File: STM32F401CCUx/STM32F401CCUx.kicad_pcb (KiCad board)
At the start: 2 copper layers, 46 x 64.5 mm, 60 parts, among them J1 Conn_01x04, J2 Power_Conn, J3 SWD, J4 USB_C_Receptacle_USB2.0, Q1 AO3401A, SW1 SW_SPDT, U1 MSM38A2718Z9BM3, U2 EUP3458, U3 LM321, U4 STM32F401CCUx, U5 USBLC6-2SC6, Y1 25MHz

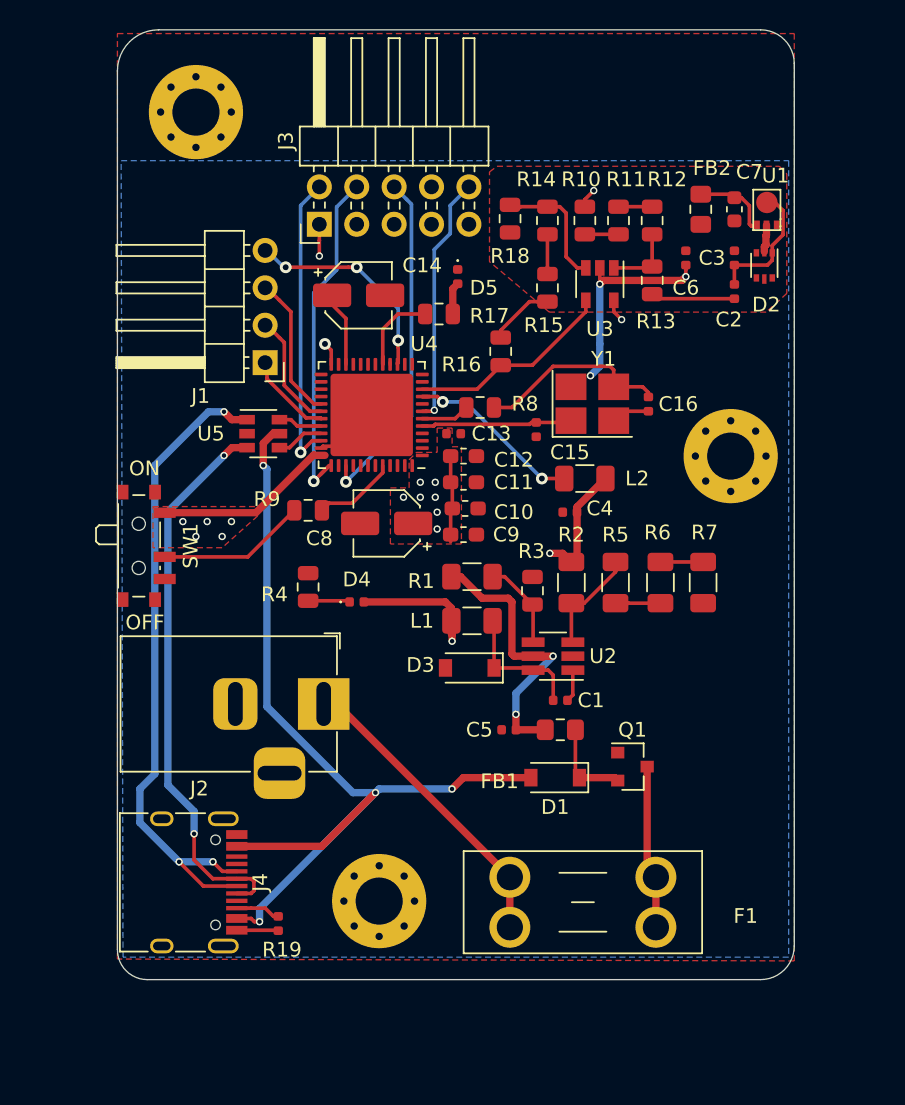
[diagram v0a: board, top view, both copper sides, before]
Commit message: Updated PCB
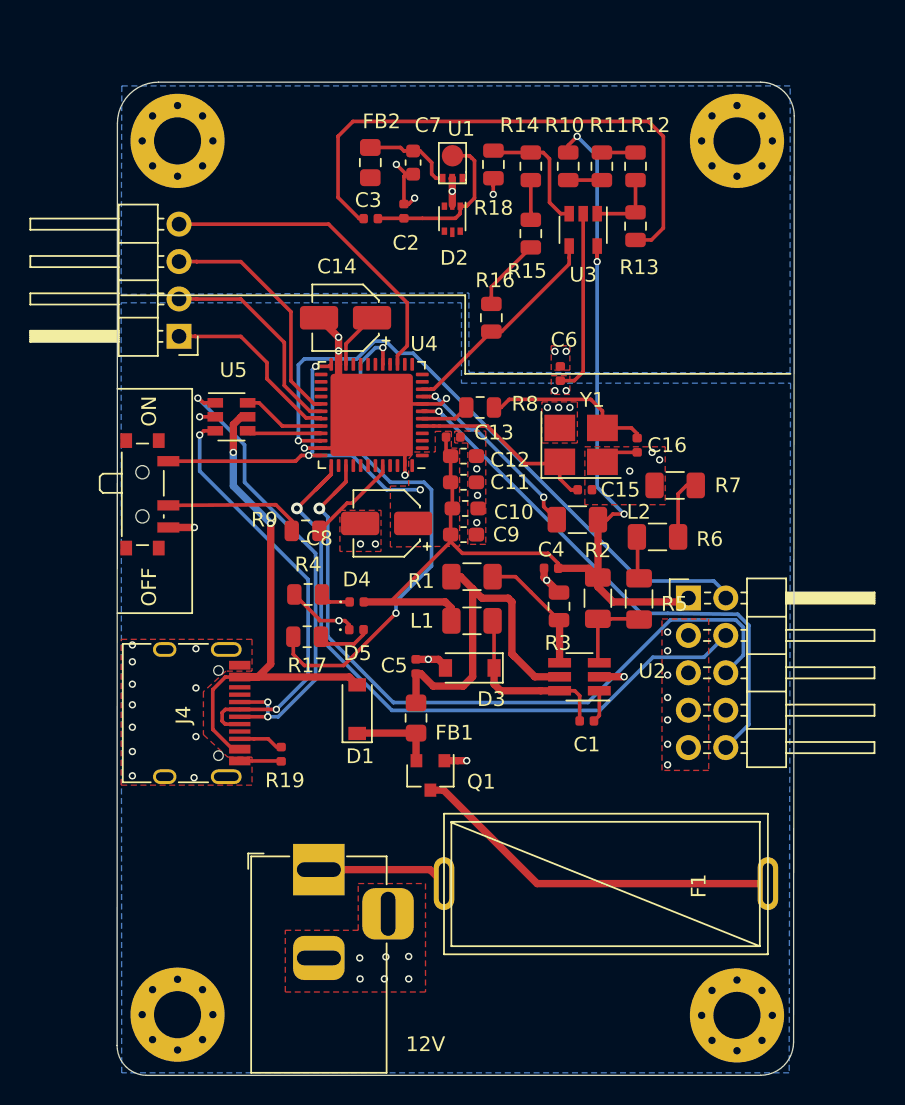
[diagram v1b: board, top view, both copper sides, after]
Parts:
- removed the REF** at (95.2, 82.0)
- removed the REF** at (131.6, 105.4)
- removed the REF** at (107.7, 135.6)
- added REF**: MountingHole_3.2mm_M3_Pad_Via, MountingHole:MountingHole_3.2mm_M3_Pad_Via, F.Cu at (94.0, 143.3)
- added REF**: MountingHole_3.2mm_M3_Pad_Via, MountingHole:MountingHole_3.2mm_M3_Pad_Via, F.Cu at (132.0, 143.4)
- added REF**: MountingHole_3.2mm_M3_Pad_Via, MountingHole:MountingHole_3.2mm_M3_Pad_Via, F.Cu at (132.0, 84.0)
- added REF**: MountingHole_3.2mm_M3_Pad_Via, MountingHole:MountingHole_3.2mm_M3_Pad_Via, F.Cu at (94.0, 84.0)
- F1: footprint Fuse:Fuseholder_Blade_Mini_Keystone_3568 -> Fuse_holder:FUSE-TH_L22.6-W9.0
- moved J3 35.7 mm to (128.7, 115.0), turned to 0 degrees
- moved C2 25.2 mm to (107.1, 89.3), turned to 0 degrees
- moved D5 24.9 mm to (106.2, 117.2), turned to 0 degrees
- moved R17 23.7 mm to (102.8, 117.7)
- moved FB2 22.7 mm to (107.1, 85.5)
- moved C3 22.7 mm to (109.4, 88.8)
- moved C7 22.1 mm to (110.0, 85.5)
- moved U1 21.6 mm to (113.6, 84.1)
- moved D2 21.4 mm to (112.7, 89.3)
- moved D1 14.2 mm to (106.2, 122.6), turned to 90 degrees
- moved Q1 13.7 mm to (111.2, 127.1), turned to 270 degrees
- moved C6 11.6 mm to (120.0, 99.8)
- moved J4 11.5 mm to (94.2, 122.9)
- moved R19 11.5 mm to (101.0, 125.7)
- moved J2 11.3 mm to (103.6, 133.5), turned to 90 degrees
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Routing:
- net +3V3: track 41.4 -> 103.0 mm, vias 18 -> 6
- net GND: track 24.2 -> 60.2 mm, vias 3 -> 49
- net CODEC_OUT: track 5.72 -> 38.3 mm
- net LED_STATUS: track 6.24 -> 34.4 mm, vias 0 -> 2
- net +5V: track 64.7 -> 37.2 mm, vias 4 -> 2
- net SWO: track 23.7 -> 49.9 mm
- net SWDIO: track 20.3 -> 43.9 mm
- net SWCLK: track 23.7 -> 47.2 mm
- net NRST: track 17.0 -> 37.4 mm
- net Net-(F1-Pad1): track 11.2 -> 25.6 mm
- net USB_CONN_D-: track 45.2 -> 32.9 mm
- net +12V: track 20.9 -> 8.89 mm
- net USB_CONN_D+: track 38.1 -> 29.4 mm
- net PWM: track 14.4 -> 22.2 mm, vias 3 -> 0
- net PA8: track 9.69 -> 16.4 mm
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- added copper zone on B.Cu, net GND
- added copper zone on B.Cu, net MSM_GND
- removed copper zone on B.Cu, net +3V3
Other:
- board size 46 x 64.5 mm -> 46 x 67.5 mm
- board text added: "12V"
